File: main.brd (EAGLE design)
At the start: 49.7 x 43.7 mm, 18 parts, among them IC1 PCF8574P, U1 BMP280

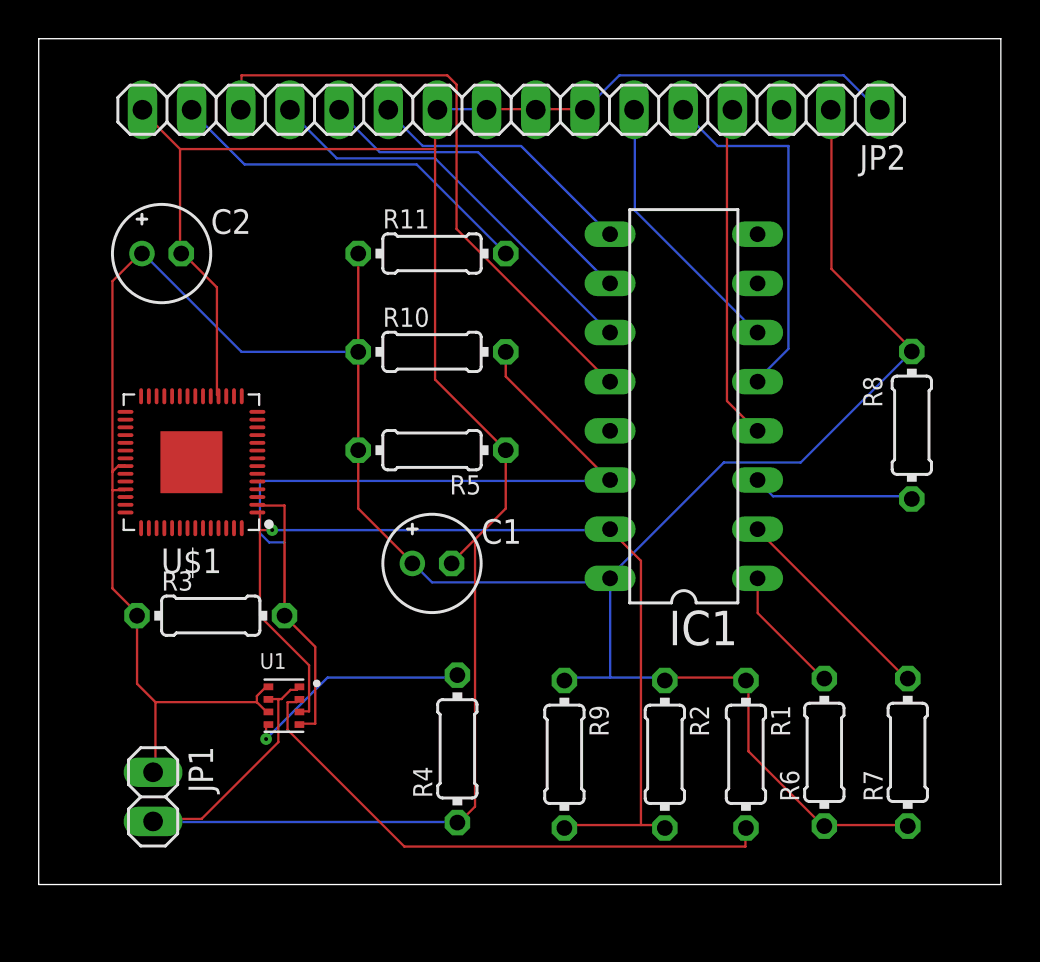
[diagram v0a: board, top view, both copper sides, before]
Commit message: Update files
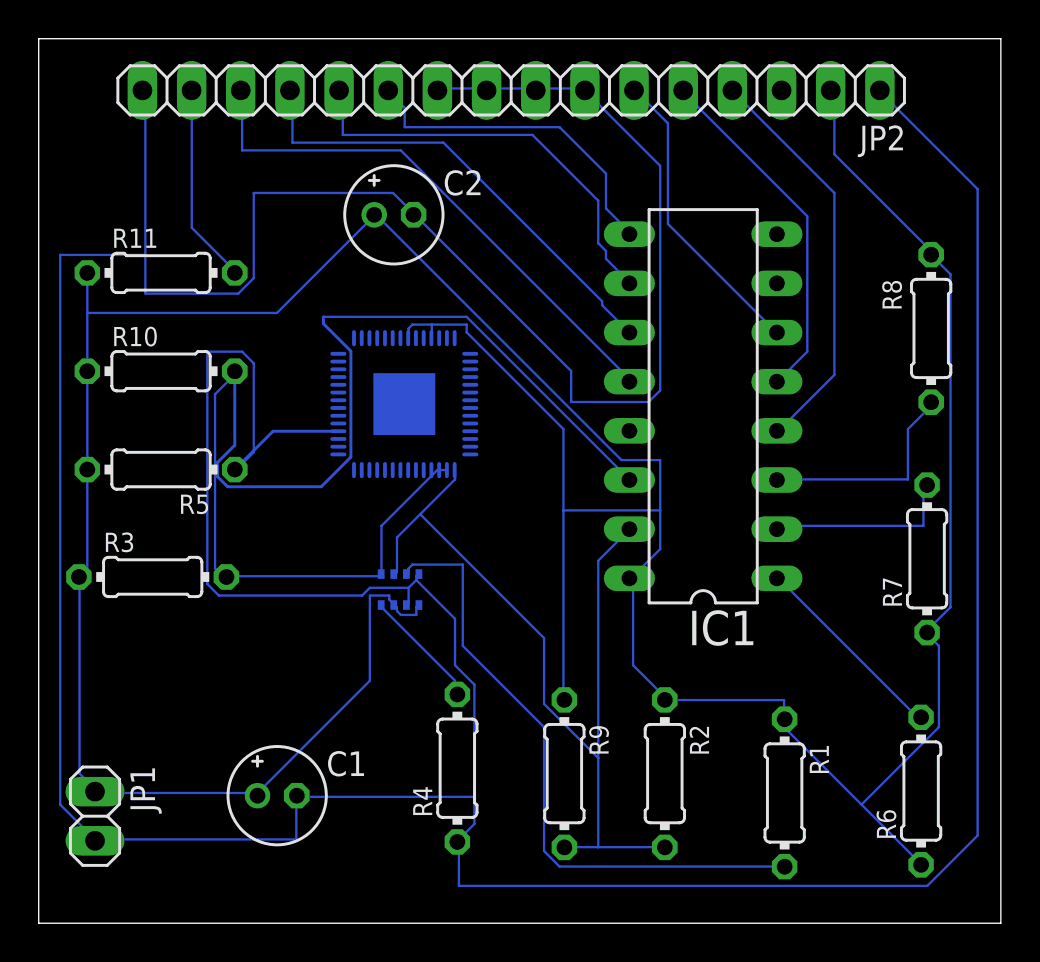
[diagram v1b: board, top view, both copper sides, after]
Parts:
- moved C1 14.4 mm to (97.4, 24.1)
- moved R10 14.0 mm to (91.4, 46.0)
- moved R11 14.0 mm to (91.4, 51.1)
- moved R5 14.0 mm to (91.4, 40.9)
- moved C2 12.2 mm to (103.4, 54.1)
- moved U$1 11.4 mm to (104.0, 44.3), flipped to the bottom, turned to 90 degrees
- moved R7 10.0 mm to (131.0, 36.3)
- moved U1 8.49 mm to (103.8, 34.7), flipped to the bottom, turned to 90 degrees
- moved R6 5.39 mm to (130.7, 24.3)
- moved R8 5.10 mm to (131.2, 48.2)
- moved R3 3.61 mm to (91.0, 35.4)
- moved JP1 3.16 mm to (88.0, 23.0)
- moved R1 2.83 mm to (123.6, 24.2)
- moved IC1 1.00 mm to (119.4, 44.2)
- moved JP2 1.00 mm to (109.5, 60.5)
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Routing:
- net GND: track 123.3 -> 255.2 mm
- net VCC: track 141.6 -> 193.4 mm
- net SCL: track 49.1 -> 67.3 mm
- net N$14: track 19.4 -> 10.3 mm
- net SDA: track 51.4 -> 45.4 mm, vias 1 -> 0
- net SDO: track 12.1 -> 6.25 mm, vias 1 -> 0
- net N$3: track 17.7 -> 22.0 mm
- net N$9: track 6.63 -> 10.5 mm
- net N$5: track 17.4 -> 21.0 mm
- net N$1: track 31.8 -> 28.2 mm
- net CSB: track 29.2 -> 32.5 mm
- net N$4: track 14.2 -> 17.3 mm
- net N$2: track 21.3 -> 24.4 mm
- net N$11: track 8.46 -> 11.3 mm
- net N$8: track 14.2 -> 15.6 mm
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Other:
- board size 49.7 x 43.7 mm -> 49.7 x 45.7 mm
